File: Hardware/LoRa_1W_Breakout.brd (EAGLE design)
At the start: 43.2 x 53.3 mm, 71 parts, among them U4 E19-915M30S

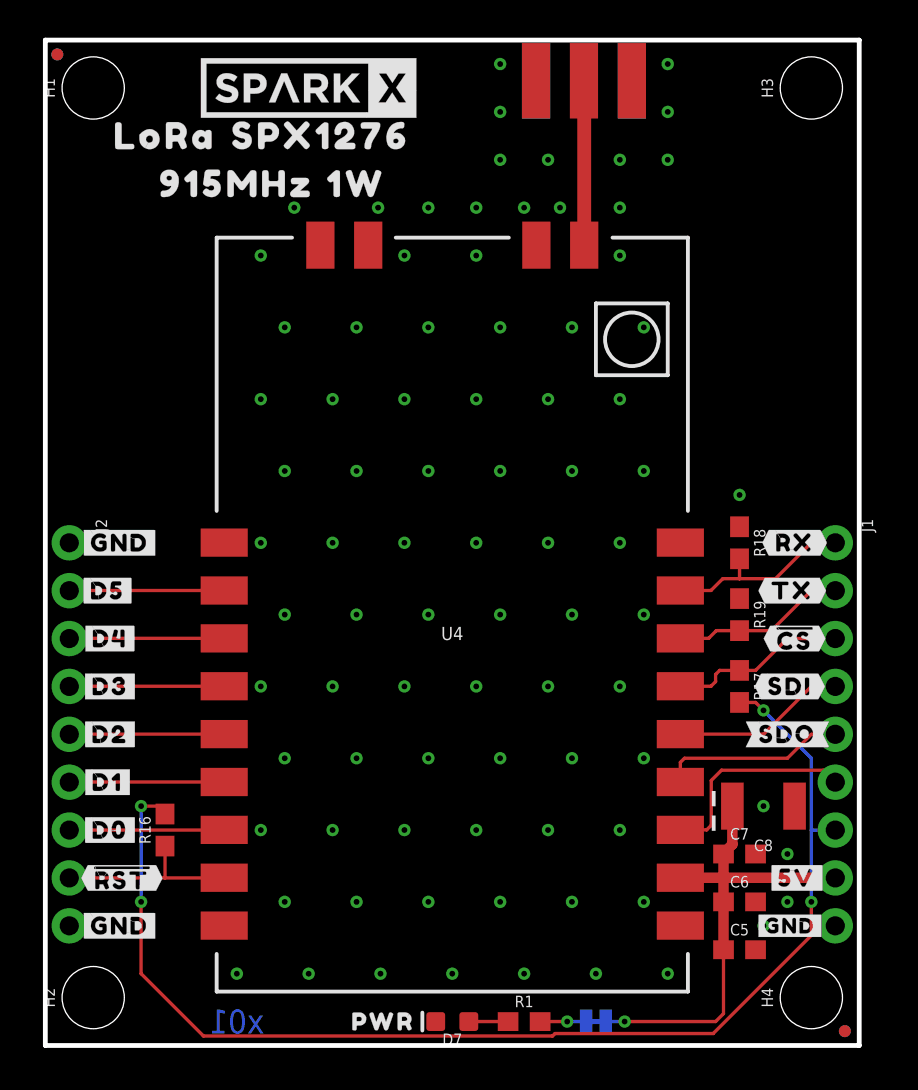
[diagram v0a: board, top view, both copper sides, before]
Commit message: Update to x02
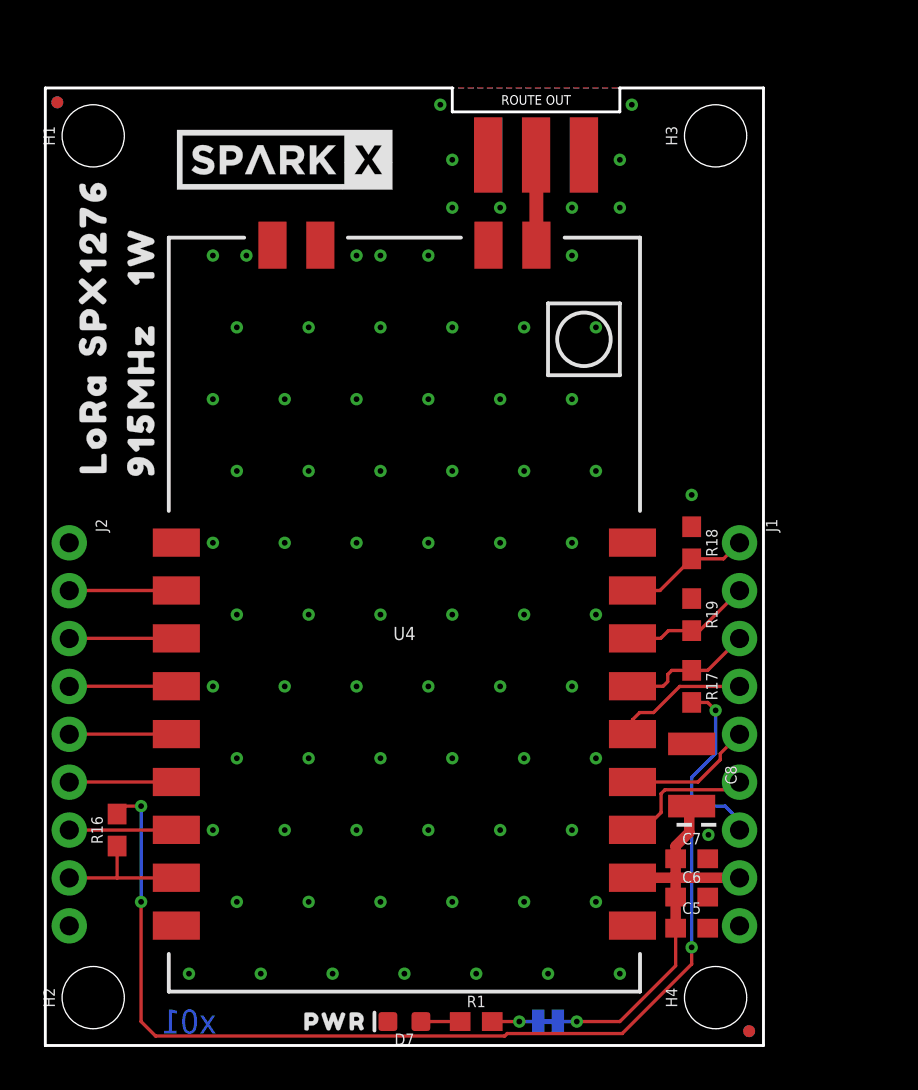
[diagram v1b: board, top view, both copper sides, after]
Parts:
- removed U$17: (no value), output:#RX#1
- removed U$20: (no value), output:#5V#1
- removed U$21: (no value), output:#TX#0
- removed U$22: (no value), output:#SDI#4
- removed U$24: (no value), output:#SDO#3
- removed U$25: (no value), output:##CS##5
- removed U$30: (no value), output:#GND#0
- removed U$31, U$32: (no value), output:#GND#8
- removed U$33: (no value), output:##RST##0
- removed U$34: (no value), output:#D0#1
- removed U$35: (no value), output:#D1#2
- removed U$36: (no value), output:#D2#3
- removed U$38: (no value), output:#D3#4
- removed U$41: (no value), output:#D4#5
- removed U$42: (no value), output:#D5#6
- C8: value 68uF -> 47uF
- moved U$67 15.7 mm to (2.54, 33.0), turned to 90 degrees
- moved U$69 13.9 mm to (2.54, 41.3), turned to 90 degrees
- moved U$7 12.5 mm to (5.08, 34.3), turned to 90 degrees
- moved U$27 12.0 mm to (5.08, 41.9), turned to 90 degrees
- moved H3 5.68 mm to (35.6, 48.3)
- moved U$52 5.08 mm to (34.2, 6.35)
- moved U$62 5.08 mm to (34.2, 14.0)
- moved FD1 5.08 mm to (37.3, 0.76)
- moved FD3 5.08 mm to (37.3, 0.76)
- moved H4 5.08 mm to (35.6, 2.54)
- moved J1 5.08 mm to (36.8, 26.7)
- moved U$43 5.08 mm to (34.8, 8.89)
- moved U$44 5.08 mm to (34.3, 11.4)
- moved U$45 5.08 mm to (34.3, 16.5)
- moved U$46 5.08 mm to (34.4, 19.1)
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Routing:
- net LORA_RF: track 8.73 -> 4.79 mm
- net LORA_SCK: track 11.2 -> 7.32 mm
- net 5V: track 25.9 -> 22.0 mm
- net LORA_RXEN: track 10.3 -> 6.73 mm
- net LORA_CIPO: track 9.88 -> 6.92 mm
- net LORA_D5: track 8.22 -> 5.68 mm
- net LORA_D4: track 8.22 -> 5.68 mm
- net LORA_D1: track 8.22 -> 5.68 mm
- net LORA_D0: track 9.56 -> 7.02 mm
- net LORA_!RST!: track 11.3 -> 8.71 mm
- net LORA_D3: track 8.22 -> 5.68 mm
- net LORA_D2: track 8.22 -> 5.68 mm
- net LORA_!CS!: track 9.49 -> 6.95 mm
- net LORA_TXEN: track 9.27 -> 6.73 mm
- net 3.3V: track 65.2 -> 62.8 mm
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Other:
- board size 43.2 x 53.3 mm -> 38.1 x 50.8 mm
- board text added: "ROUTE OUT"
